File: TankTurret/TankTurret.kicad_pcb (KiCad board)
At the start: 2 copper layers, 35 x 60 mm, 56 parts, among them J1 Conn_01x04_Socket, J2 USB_C_Receptacle_USB2.0_16P, J3 Camera, Q1 MMBT3904, SW1 SW_Push, SW2 SW_Push, U1 ESP32-S3-WROOM-1, U2 TLV70028_SOT353, U3 TLV70012_SOT23-5

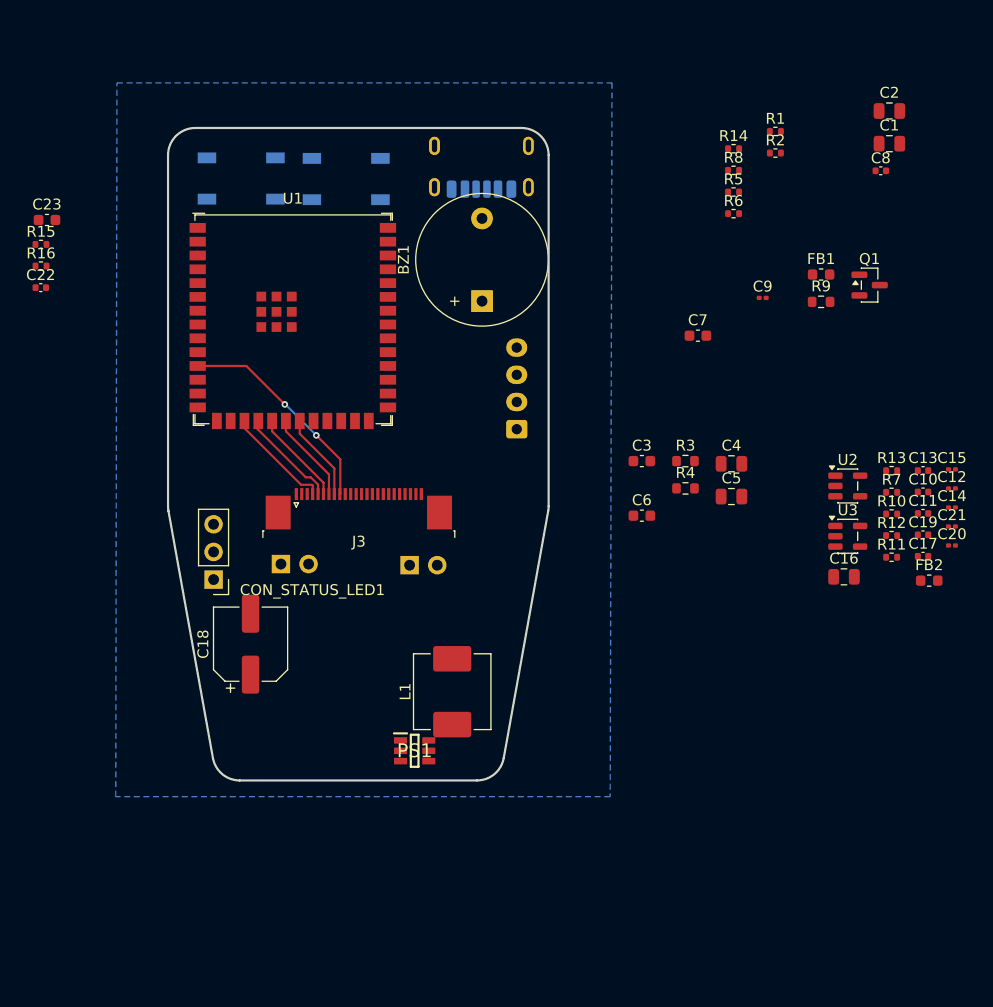
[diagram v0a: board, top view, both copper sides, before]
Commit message: Signed-off-by: SMAUG\Pete <pwbrophy@gmail.com>
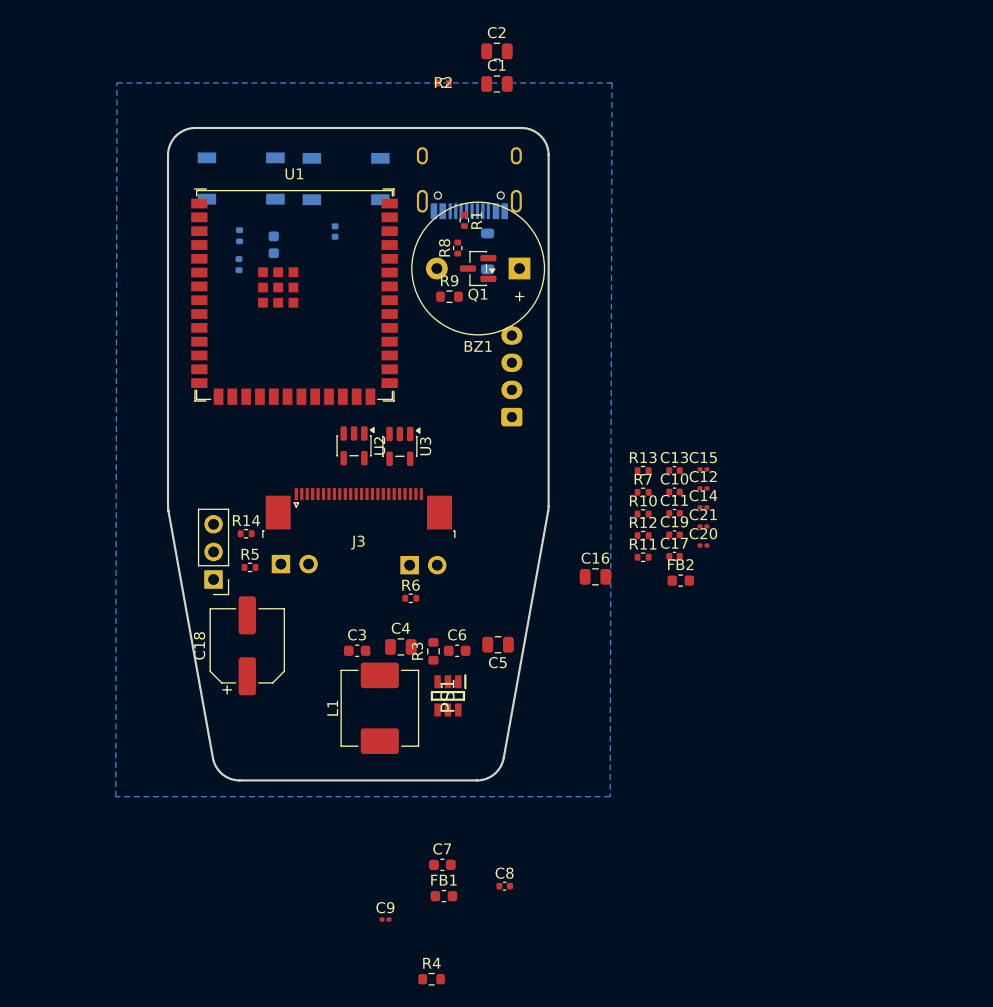
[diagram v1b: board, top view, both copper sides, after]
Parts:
- added D1: D_Schottky, Diode_SMD:D_SOD-123, B.Cu at (83.2, 52.6)
- C22, C23, R15, R16: moved to B.Cu
- J2: footprint Connector_USB:USB_C_Receptacle_HRO_TYPE-C-31-M-17 -> Connector_USB:USB_C_Receptacle_HRO_TYPE-C-31-M-12
- moved C8 74.3 mm to (84.8, 111.0)
- moved C9 66.9 mm to (73.8, 114.1)
- moved FB1 66.9 mm to (79.2, 111.9)
- moved R14 57.1 mm to (61.0, 78.6)
- moved R5 56.3 mm to (61.4, 81.7)
- moved C7 54.0 mm to (79.1, 109.0)
- moved R4 50.8 mm to (78.1, 119.6)
- moved R6 46.2 mm to (76.1, 84.5)
- moved U2 45.6 mm to (70.9, 70.5), turned to -90 degrees
- moved U3 42.0 mm to (75.1, 70.6), turned to -90 degrees
- moved C1 36.5 mm to (84.1, 37.2)
- moved C2 36.5 mm to (84.1, 34.2)
- moved Q1 36.0 mm to (82.3, 54.2), turned to 180 degrees
- moved C4 34.8 mm to (75.2, 89.0)
- moved R9 34.2 mm to (79.7, 56.8)
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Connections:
- C1 pad 1: +BATT -> +5V_USB
- C2 pad 1: +BATT -> +5V_USB
- J2 pad A9: +BATT -> +5V_USB
- J2 pad B9: +BATT -> +5V_USB
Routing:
- net /GPIO18: track 19.9 -> 0.00 mm, vias 2 -> 0
- net /GPIO9: track 9.91 -> 0.00 mm
- net /GPIO10: track 9.34 -> 0.00 mm
- net /GPIO11: track 8.68 -> 0.00 mm
- net /GPIO12: track 8.36 -> 0.00 mm
- net /GPIO13: track 8.04 -> 0.00 mm
